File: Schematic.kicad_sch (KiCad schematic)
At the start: 56 parts, among them J1 Screw_Terminal_01x04, Q1 HY1707, Q2 HY1707, Q3 S8050, Q4 2N2222, U1 UC2843A, U2 SFH618A-5, U3 TL431LP

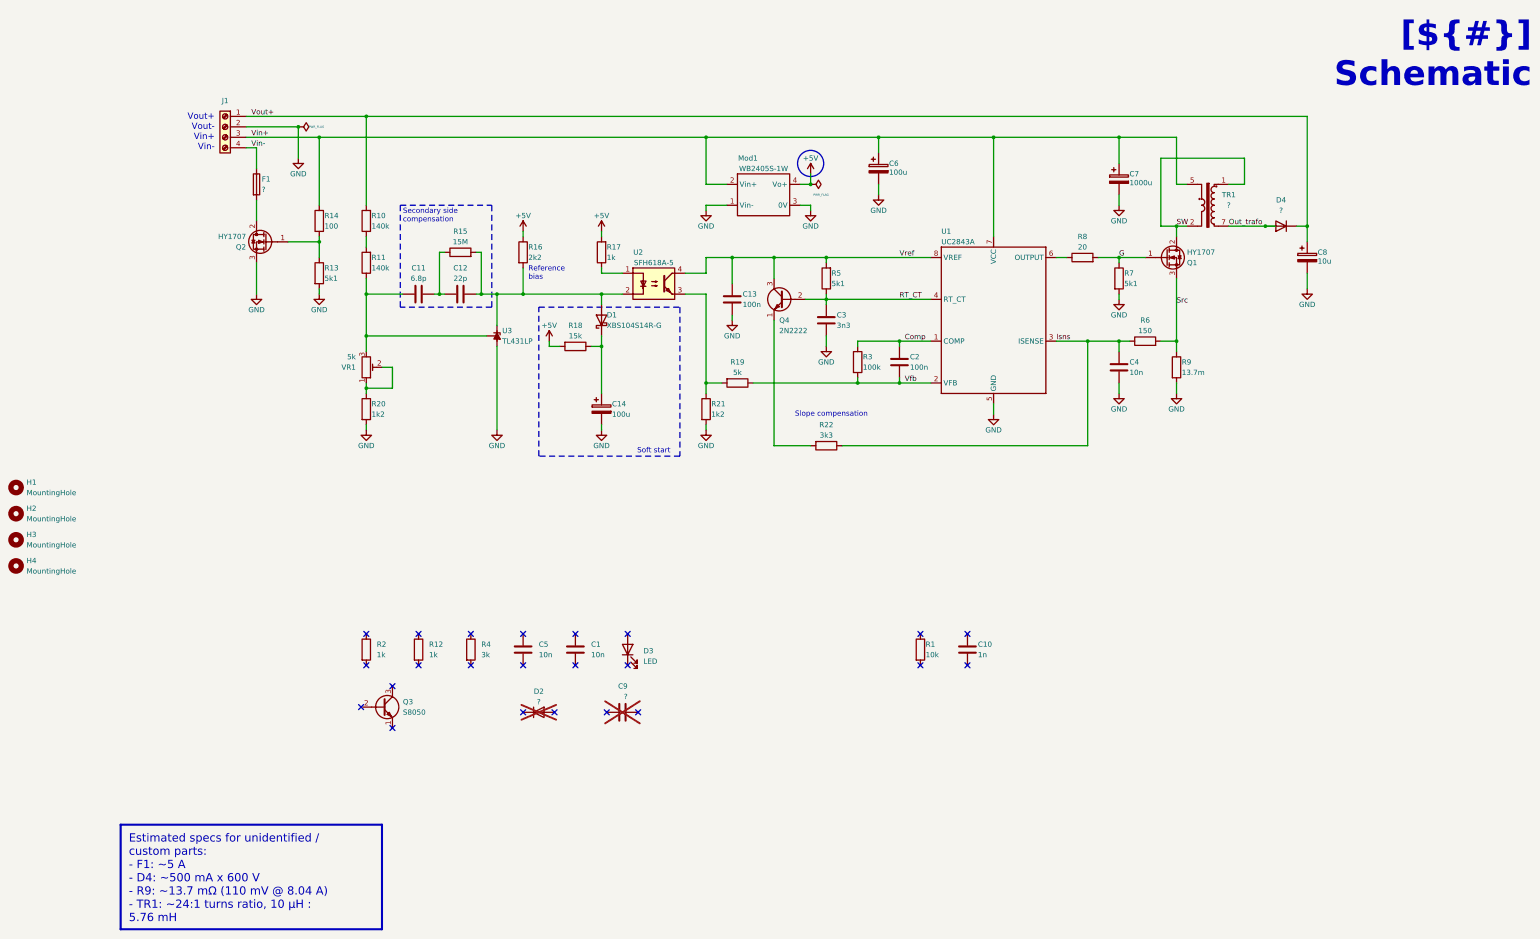
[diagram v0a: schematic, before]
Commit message: First working prototype - still not isolated
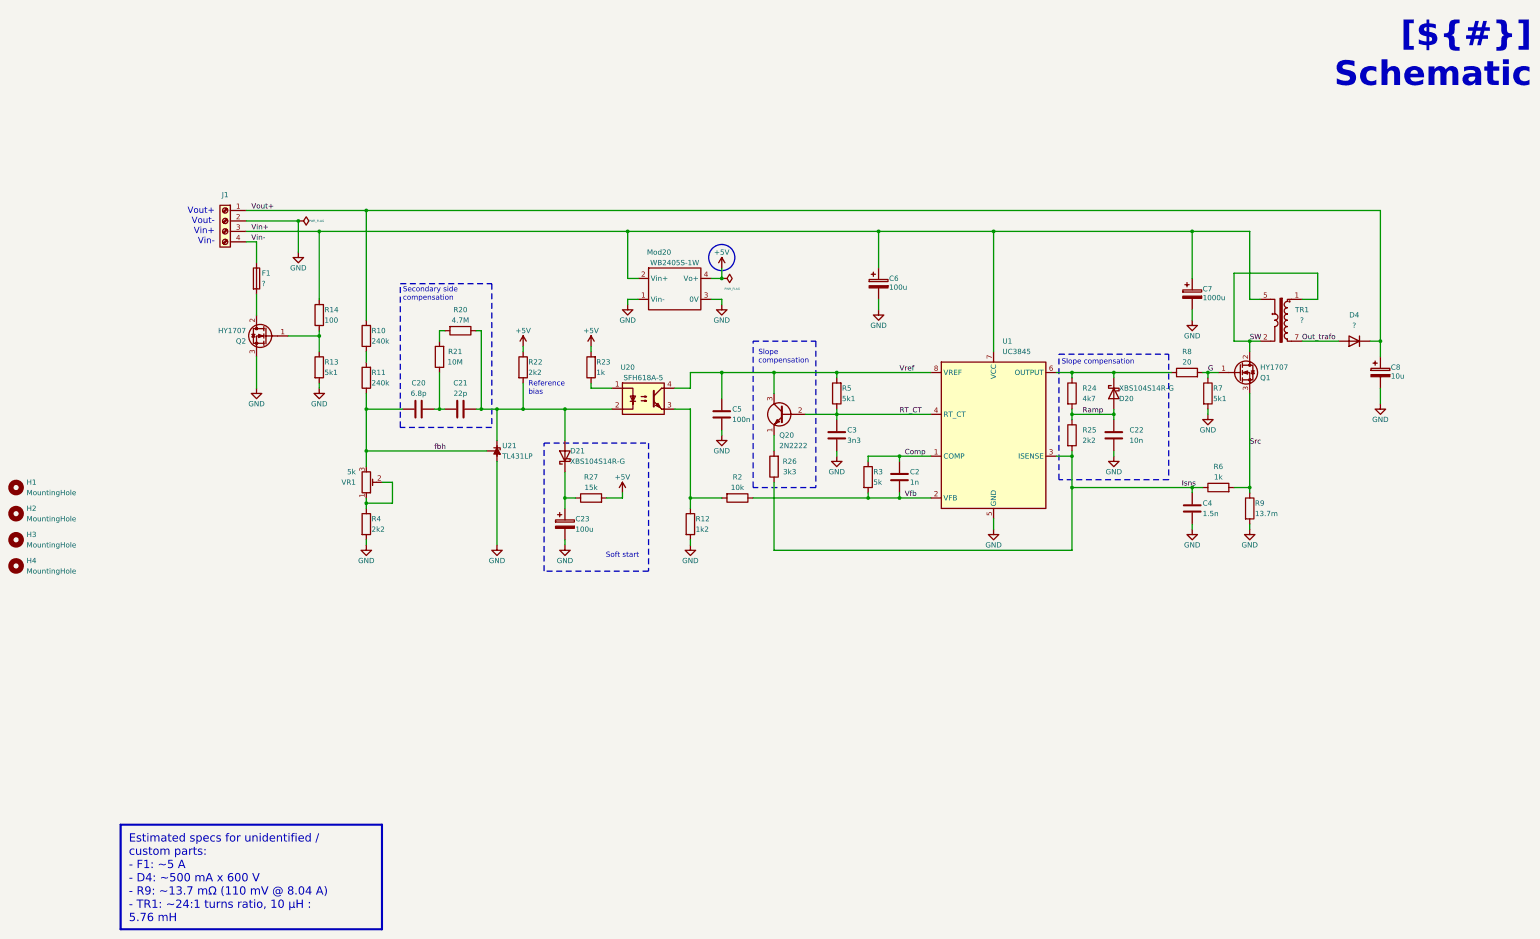
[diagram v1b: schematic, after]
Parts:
- removed C1, C5: 10n, Capacitor_THT:C_Rect_L7.0mm_W2.0mm_P5.00mm, symbol Device:C
- removed C10: 1n, Capacitor_THT:C_Disc_D3.8mm_W2.6mm_P2.50mm, symbol Device:C
- removed C9: ?, Capacitor_THT:C_Rect_L7.0mm_W2.0mm_P5.00mm, symbol Device:C
- removed D2: ?, Diode_THT:D_A-405_P7.62mm_Horizontal, symbol Device:D
- removed D3: LED, LED_THT:LED_D3.0mm, symbol Device:LED
- removed Q3: S8050, Package_TO_SOT_THT:TO-92_Inline_Wide, symbol Transistor_BJT:S8050
- removed R1: 10k, Resistor_THT:R_Axial_DIN0207_L6.3mm_D2.5mm_P2.54mm_Vertical, symbol Device:R
- removed R12, R2: 1k, Resistor_THT:R_Axial_DIN0207_L6.3mm_D2.5mm_P7.62mm_Horizontal, symbol Device:R
- removed R4: 3k, Resistor_THT:R_Axial_DIN0207_L6.3mm_D2.5mm_P7.62mm_Horizontal, symbol Device:R
- removed U1: UC2843A, Package_DIP:DIP-8_W7.62mm, symbol personal:UC2843AQD8R
- added C22: 10n, Capacitor_THT:C_Disc_D3.0mm_W1.6mm_P2.50mm, symbol Device:C
- added D20: XBS104S14R-G, Diode_SMD:D_SOD-123F, symbol Device:D_Schottky
- added R20: 4.7M, Resistor_THT:R_Axial_DIN0204_L3.6mm_D1.6mm_P5.08mm_Vertical, symbol Device:R
- added R24: 4k7, Resistor_THT:R_Axial_DIN0204_L3.6mm_D1.6mm_P5.08mm_Horizontal, symbol Device:R
- added R25: 2k2, Resistor_THT:R_Axial_DIN0204_L3.6mm_D1.6mm_P2.54mm_Vertical, symbol Device:R
- added U1: UC3845, Package_DIP:DIP-8_W7.62mm, symbol personal:UC3845
- C2: value 100n -> 1n
- C20: renamed from C11; footprint Capacitor_THT:C_Disc_D7.5mm_W5.0mm_P5.00mm -> Capacitor_THT:C_Disc_D7.5mm_W5.0mm_P7.50mm
- C4: value 10n -> 1.5n
- R10, R11: value 140k -> 240k
- R2: renamed from R19; value 5k -> 10k
- R21: renamed from R15; value 15M -> 10M; footprint Resistor_THT:R_Axial_DIN0207_L6.3mm_D2.5mm_P5.08mm_Vertical -> Resistor_THT:R_Axial_DIN0204_L3.6mm_D1.6mm_P2.54mm_Vertical
- R23: renamed from R17; footprint Resistor_THT:R_Axial_DIN0204_L3.6mm_D1.6mm_P5.08mm_Horizontal -> Resistor_THT:R_Axial_DIN0204_L3.6mm_D1.6mm_P7.62mm_Horizontal
- R3: value 100k -> 5k
- R4: renamed from R20; value 1k2 -> 2k2
- R6: value 150 -> 1k
- renumbered C12 to C21, C14 to C23, C13 to C5, D1 to D21, Mod1 to Mod20, Q4 to Q20, R21 to R12, R16 to R22, R22 to R26, R18 to R27, U2 to U20, U3 to U21
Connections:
- net Comp: now also U1.1 (COMP)
- net GND: now also C22.2, U1.5 (GND)
- net Isns: now also R25.2, U1.3 (ISENSE)
- net RT_CT: now also U1.4 (RT_CT)
- net Vfb: now also U1.2 (VFB)
- net Vin+: now also U1.7 (VCC)
- net Vref: now also U1.8 (VREF)
- net at C21.2, D21.2 (A), R22.2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: now also R20.1; no longer R21.2
- net fbh: now reaches C20.1, R11.1, U21.1 (REF), VR1.3
- net at R8.1: now also D20.1 (K), R24.1, U1.6 (OUTPUT)
- new net: R20.2, R21.2
- new net Ramp: C22.1, D20.2 (A), R24.2, R25.1
- no-connect marks 23 -> 0
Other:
- moved on the sheet: C2, C20, C21, C23, C3, C4, C5, C6, C7, C8, D21, D4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
